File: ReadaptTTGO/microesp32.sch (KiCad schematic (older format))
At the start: 1 part, among them U2 ESP32

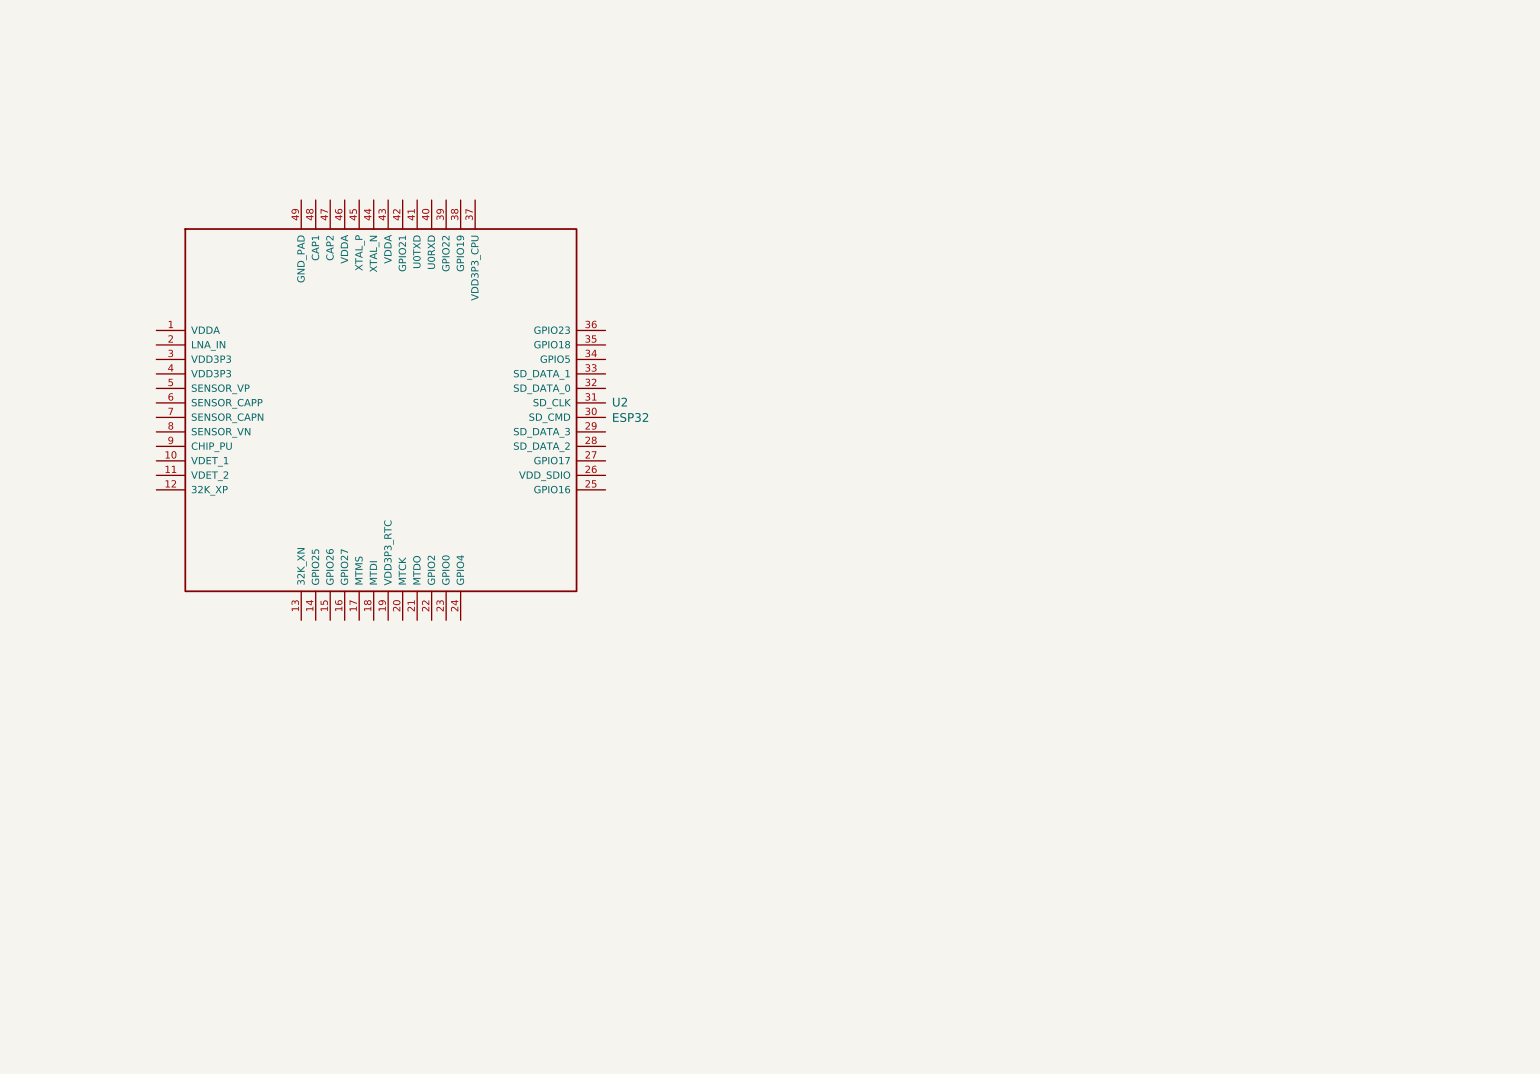
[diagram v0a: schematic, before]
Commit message: Primer aproximacion.
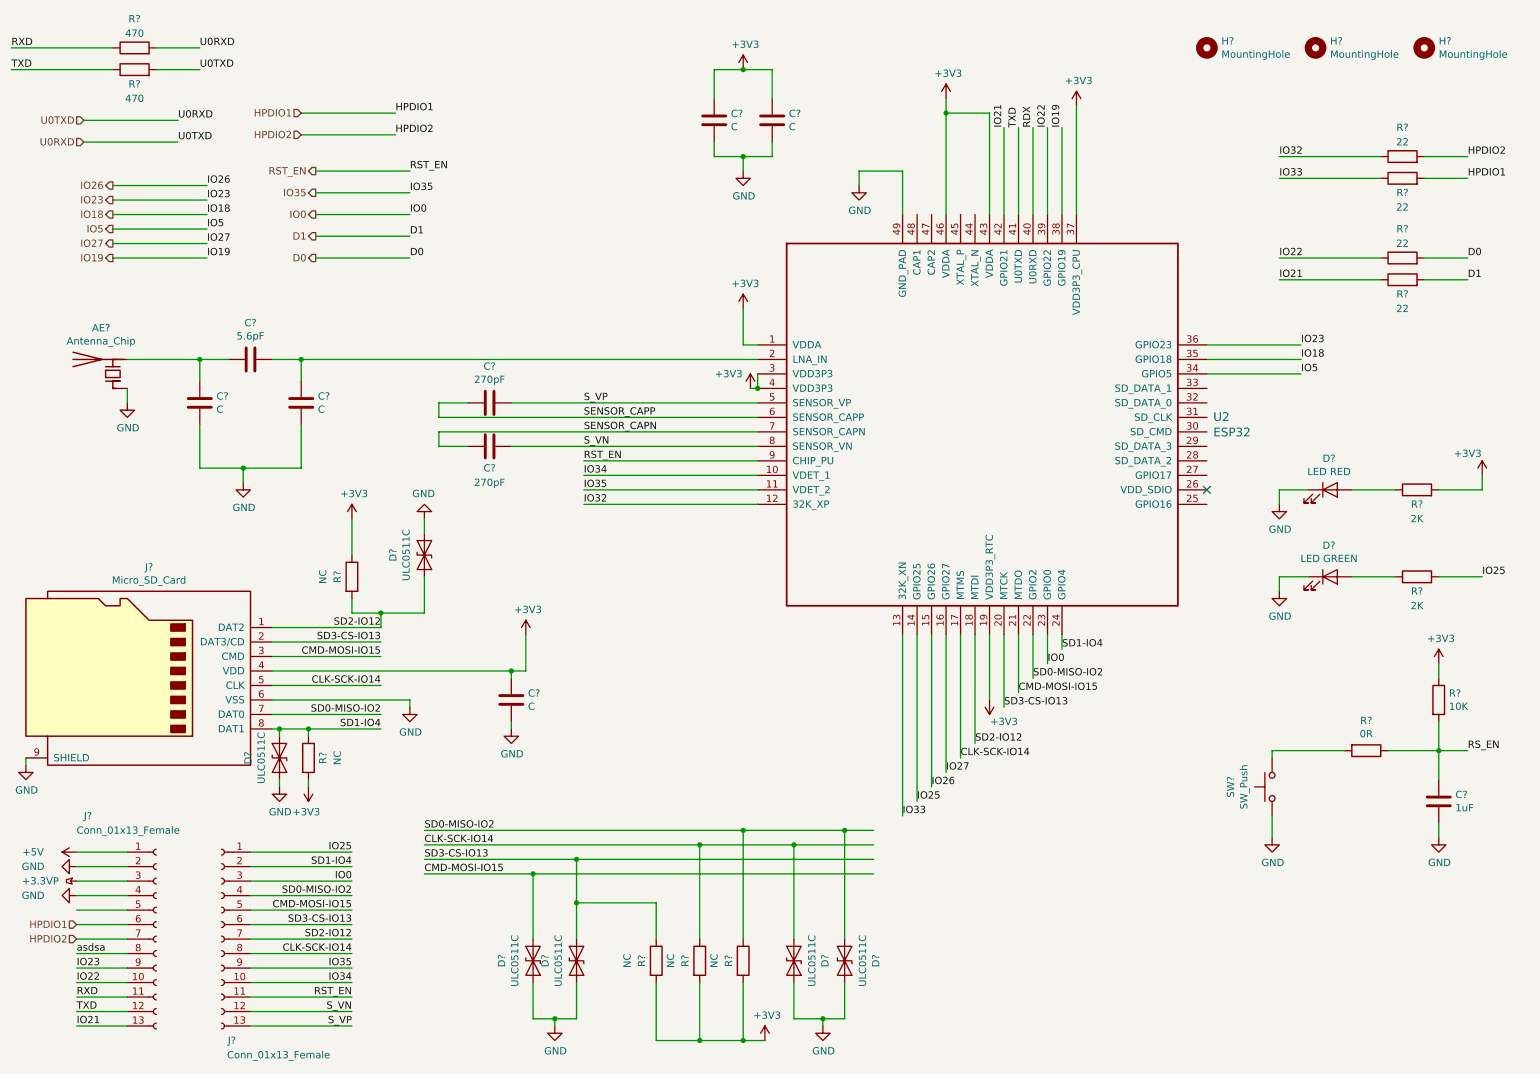
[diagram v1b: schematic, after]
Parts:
- added AE?: Antenna_Chip, symbol Device:Antenna_Chip
- added C? (x5): C, symbol Device:C
- added C?: 5.6pF, symbol Device:C
- added C? (x2): 270pF, symbol Device:C
- added C?: 1uF, symbol Device:C
- added D?: LED RED, symbol Device:LED
- added D?: LED GREEN, symbol Device:LED
- added D? (x6): ULC0511C, symbol Device:D_TVS
- added H? (x3): MountingHole, symbol Mechanical:MountingHole
- added J? (x2): Conn_01x13_Female, symbol Connector:Conn_01x13_Female
- added J?: Micro_SD_Card, symbol Connector:Micro_SD_Card
- added R?: 10K, symbol Device:R
- added R?: 0R, symbol Device:R
- added R? (x2): 470, symbol Device:R
- added R? (x4): 22, symbol Device:R
- added R? (x2): 2K, symbol Device:R
- added R? (x5): NC, symbol Device:R
- added SW?: SW_Push, symbol Switch:SW_Push
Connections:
- net +3V3: now reaches U2.1 (VDDA)
- net +3V3: now also U2.19 (VDD3P3_RTC), U2.3 (VDD3P3), U2.37 (VDD3P3_CPU), U2.4 (VDD3P3), U2.43 (VDDA), U2.46 (VDDA), C?.1, C?.1, C?.1, J?.4 (VDD), R?.1, R?.1, R?.2, R?.2, R?.2, R?.2, R?.2
- net IO34: now reaches U2.10 (VDET_1)
- net IO34: now also J?.10 (Pin_10)
- net IO35: now reaches U2.11 (VDET_2)
- net IO35: now also J?.9 (Pin_9)
- net IO32: now reaches U2.12 (32K_XP)
- net IO32: now also R?.1
- net IO33: now reaches U2.13 (32K_XN)
- net IO33: now also R?.1
- net IO25: now reaches U2.14 (GPIO25)
- net IO25: now also J?.1 (Pin_1), R?.2
- net IO26: now reaches U2.15 (GPIO26)
- net IO27: now reaches U2.16 (GPIO27)
- net CLK-SCK-IO14: now reaches U2.17 (MTMS)
- net CLK-SCK-IO14: now also D?.1 (A1), J?.5 (CLK), J?.8 (Pin_8), R?.1
- net SD2-IO12: now reaches U2.18 (MTDI)
- net SD2-IO12: now also D?.1 (A1), J?.1 (DAT2), J?.7 (Pin_7), R?.2
- net at U2.2 (LNA_IN): now also C?.1, C?.1
- net SD3-CS-IO13: now reaches U2.20 (MTCK)
- net SD3-CS-IO13: now also D?.2 (A2), J?.2 (DAT3/CD), J?.6 (Pin_6), R?.1
- net CMD-MOSI-IO15: now reaches U2.21 (MTDO)
- net CMD-MOSI-IO15: now also D?.2 (A2), J?.3 (CMD), J?.5 (Pin_5)
- net SD0-MISO-IO2: now reaches U2.22 (GPIO2)
- net SD0-MISO-IO2: now also D?.1 (A1), J?.4 (Pin_4), J?.7 (DAT0), R?.1
- net IO0: now reaches U2.23 (GPIO0)
- net IO0: now also J?.3 (Pin_3)
- net SD1-IO4: now reaches U2.24 (GPIO4)
- net SD1-IO4: now also D?.2 (A2), J?.2 (Pin_2), J?.8 (DAT1), R?.1
- net IO5: now reaches U2.34 (GPIO5)
- net IO18: now reaches U2.35 (GPIO18)
- net IO23: now reaches U2.36 (GPIO23)
- net IO23: now also J?.9 (Pin_9)
- net IO19: now reaches U2.38 (GPIO19)
- net IO22: now reaches U2.39 (GPIO22)
- net IO22: now also J?.10 (Pin_10), R?.1
- net RDX: now reaches U2.40 (U0RXD)
- net TXD: now reaches U2.41 (U0TXD)
- net TXD: now also J?.12 (Pin_12), R?.1
- net IO21: now reaches U2.42 (GPIO21)
- net IO21: now also J?.13 (Pin_13), R?.1
- net GND: now reaches U2.49 (GND_PAD)
- net GND: now also AE?.1 (FEED), C?.2, C?.2, C?.2, C?.2, C?.2, C?.2, D?.1 (A1), D?.1 (A1), D?.1 (A1), D?.1 (K), D?.1 (K), D?.2 (A2), D?.2 (A2), D?.2 (A2), J?.2 (Pin_2), J?.4 (Pin_4), J?.6 (VSS), J?.9 (SHIELD), SW?.1
- net S_VP: now reaches U2.5 (SENSOR_VP)
- net S_VP: now also C?.1, J?.13 (Pin_13)
- net SENSOR_CAPP: now reaches U2.6 (SENSOR_CAPP)
- net SENSOR_CAPP: now also C?.2
- net SENSOR_CAPN: now reaches U2.7 (SENSOR_CAPN)
- net SENSOR_CAPN: now also C?.2
- net S_VN: now reaches U2.8 (SENSOR_VN)
- net S_VN: now also C?.1, J?.12 (Pin_12)
- net RST_EN: now reaches U2.9 (CHIP_PU)
- net RST_EN: now also J?.11 (Pin_11)
- new net: AE?.2 (PCB_Trace), C?.1, C?.2
- new net: R?.2, SW?.2
- new net: D?.2 (A), R?.1 (x2)
- new net +3.3VP: J?.3 (Pin_3)
- new net +5V: J?.1 (Pin_1)
- new net D0: R?.2
- new net D1: R?.2
- new net HPDIO1: J?.6 (Pin_6), R?.2
- new net HPDIO2: J?.7 (Pin_7), R?.2
- new net RS_EN: C?.1, R?.1, R?.2
- new net RXD: J?.11 (Pin_11), R?.1
- new net U0RXD: R?.2, R?.2
- new net asdsa: J?.8 (Pin_8)
- no-connect marks 0 -> 1
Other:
- moved on the sheet: U2
